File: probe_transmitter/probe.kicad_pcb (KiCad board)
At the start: 2 copper layers, 28 x 28 mm, 39 parts, among them Q1 PMST2222, U1 ATtiny85-20M

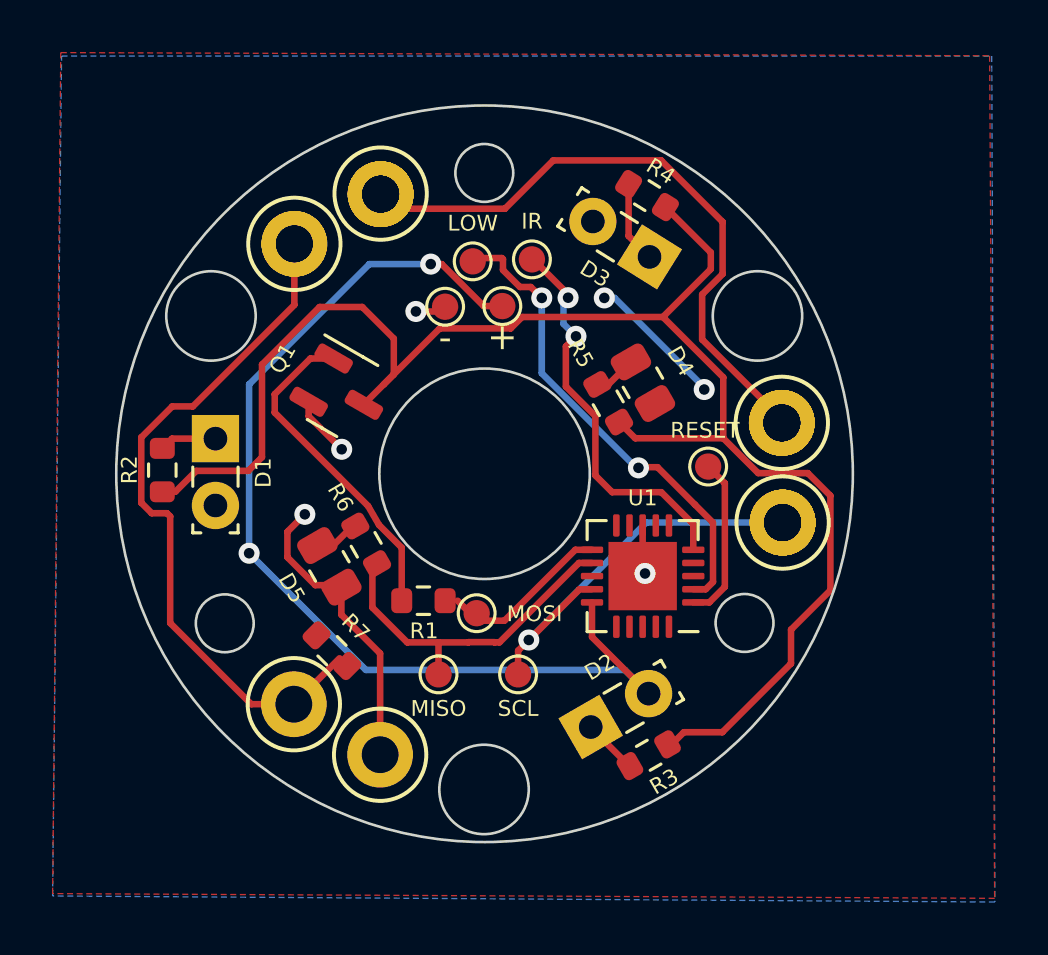
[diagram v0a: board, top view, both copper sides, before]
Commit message: - v .1.1 in prode
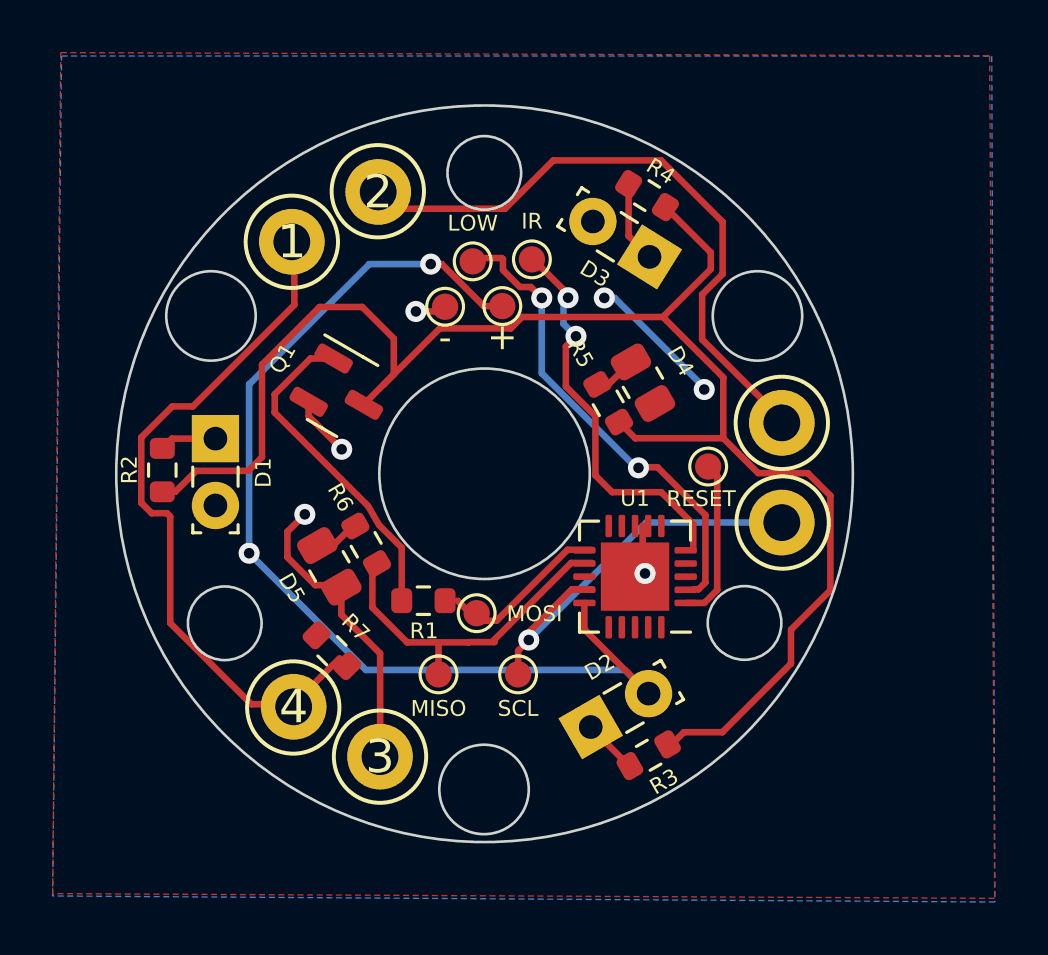
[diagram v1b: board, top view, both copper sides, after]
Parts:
- removed the ? at (111.3, 101.9) (x3)
- removed the ? at (96.0, 110.7)
- removed the ? at (96.0, 89.4) (x4)
- removed the ? at (92.8, 91.3) (x2)
- removed the ? at (111.3, 98.1) (x3)
- removed the ? at (92.8, 108.8)
- added 1: , , F.Cu at (92.7, 91.2)
- added 2: , , F.Cu at (96.0, 89.3)
- added 3: , , F.Cu at (96.0, 110.8)
- added 4: , , F.Cu at (92.7, 108.9)
- moved U1 0.29 mm to (105.7, 103.9)
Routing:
- net /PAD1: track 68.7 -> 67.9 mm
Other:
- outline, holes or cut-outs redrawn
